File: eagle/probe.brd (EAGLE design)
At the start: 21.8 x 21.8 mm, 11 parts

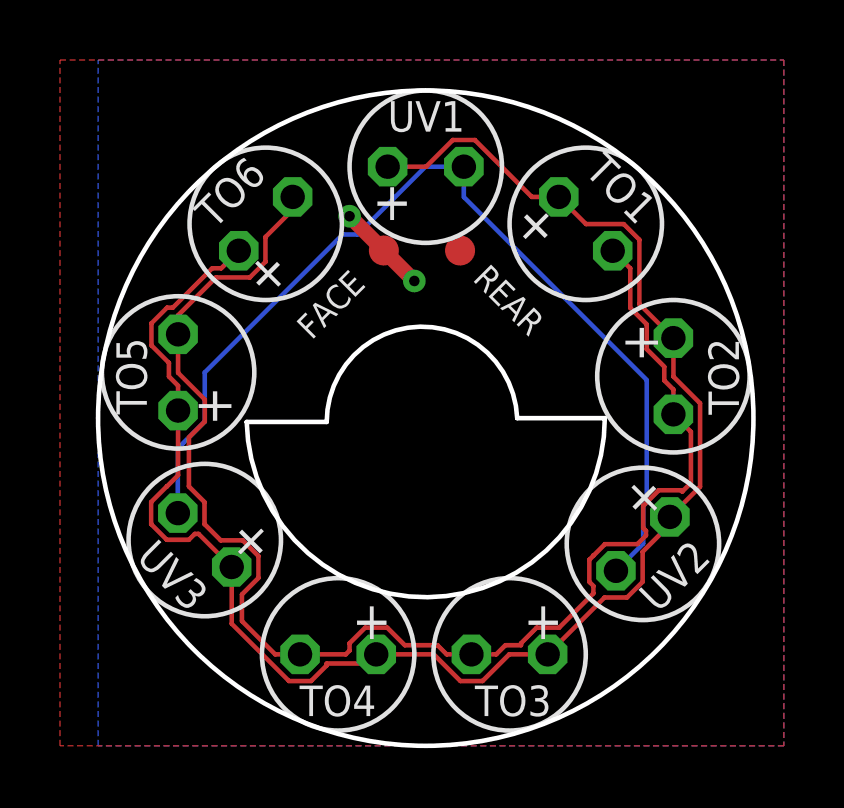
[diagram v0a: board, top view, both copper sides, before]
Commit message: new pcbs
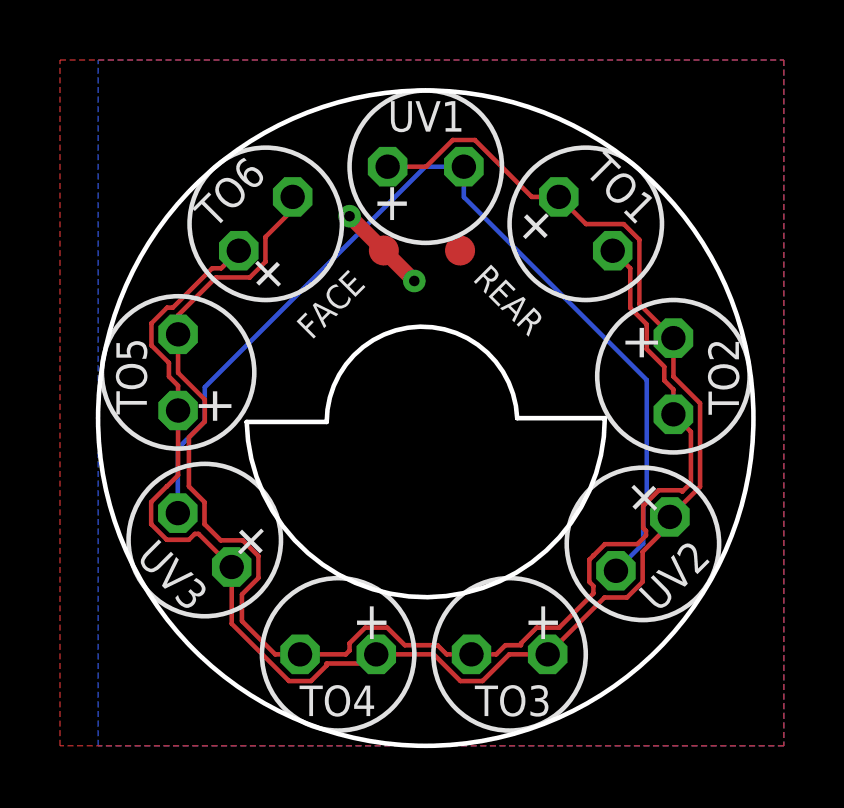
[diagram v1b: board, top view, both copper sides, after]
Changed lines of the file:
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@@
 <param name="mdViaViaSameLayer" value="6mil"/>
 <param name="mnLayersViaInSmd" value="2"/>
-<param name="mdCopperDimension" value="18mil"/>
+<param name="mdCopperDimension" value="20mil"/>
 <param name="mdDrill" value="6mil"/>
 <param name="mdSmdStop" value="0mil"/>
@@
 <wire x1="18.170025" y1="7.997259375" x2="18.170025" y2="6.740025" width="0.1524" layer="16"/>
 <wire x1="2.657971875" y1="7.756025" x2="2.657971875" y2="9.909734375" width="0.1524" layer="16"/>
-<wire x1="2.657971875" y1="9.909734375" x2="3.556" y2="10.8077625" width="0.1524" layer="16"/>
-<wire x1="3.556" y1="10.8077625" x2="3.556" y2="12.446" width="0.1524" layer="16"/>
+<wire x1="3.556" y1="10.8077625" x2="2.657971875" y2="9.909734375" width="0.1524" layer="16"/>
 <wire x1="12.192" y1="18.288" x2="12.192" y2="19.304" width="0.1524" layer="16"/>
 <wire x1="18.288" y1="8.115234375" x2="18.288" y2="12.192" width="0.1524" layer="16"/>
 <wire x1="18.288" y1="12.192" x2="12.192" y2="18.288" width="0.1524" layer="16"/>
-<wire x1="10.9092375" y1="19.304" x2="12.192" y2="19.304" width="0.1524" layer="16"/>
-<wire x1="8.1562" y1="17.0462" x2="8.6514375" y2="17.0462" width="0.1524" layer="16"/>
-<wire x1="8.6514375" y1="17.0462" x2="10.9092375" y2="19.304" width="0.1524" layer="16"/>
-<wire x1="3.556" y1="12.446" x2="8.1562" y2="17.0462" width="0.1524" layer="16"/>
+<wire x1="12.192" y1="19.304" x2="10.9092375" y2="19.304" width="0.1524" layer="16"/>
+<wire x1="3.556" y1="11.9507625" x2="3.556" y2="10.8077625" width="0.1524" layer="16"/>
+<wire x1="10.9092375" y1="19.304" x2="3.556" y2="11.9507625" width="0.1524" layer="16"/>
 </signal>
 <signal name="FACE" class="1">
